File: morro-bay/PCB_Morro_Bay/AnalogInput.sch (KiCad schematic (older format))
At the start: 136 parts, among them SW1 INPUT_RANGE_SEL_1, SW2 INPUT_RANGE_SEL_2, U5 LM2902, U6 LM2902, U7 LM2902, U8 LM2902, U9 LM2902

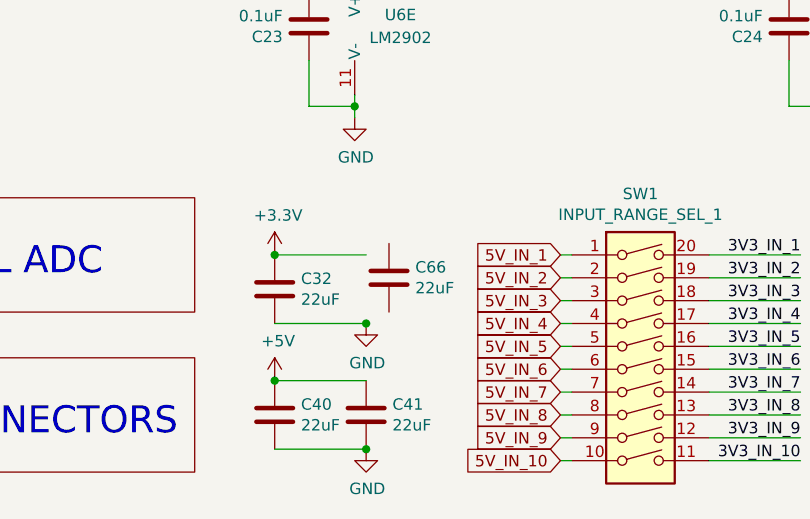
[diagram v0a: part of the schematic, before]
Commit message: Start routing
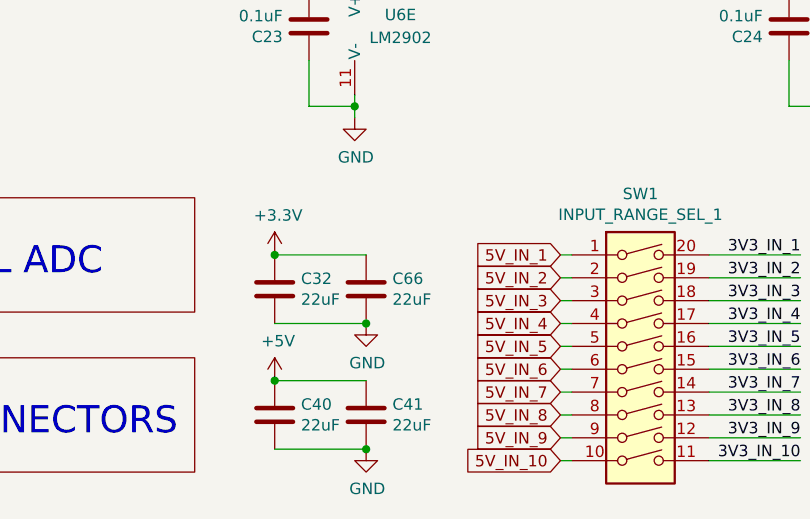
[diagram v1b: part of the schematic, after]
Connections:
- net +3V3: now also C66.1
- net GND: now also C66.2
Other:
- moved on the sheet: C66
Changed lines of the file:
@@
 Wire Wire Line
 	3000 6950 3400 6950
-Connection ~ 3400 6950
 $Comp
 L Device:C C?
@@
 L Device:C C?
 U 1 1 5E88C60F
-P 3500 6750
+P 3400 6800
 AR Path="/5E88C60F" Ref="C?"  Part="1"
 AR Path="/5E59A680/5E88C60F" Ref="C66"  Part="1"
-F 0 "C66" H 3615 6796 50  0000 L CNN
-F 1 "22uF" H 3615 6705 50  0000 L CNN
-F 2 "Capacitor_SMD:C_0805_2012Metric_Pad1.15x1.40mm_HandSolder" H 3538 6600 50  0001 C CNN
-F 3 "~" H 3500 6750 50  0001 C CNN
-F 4 "CL21A226MAQNNNE" H 3500 6750 50  0001 C CNN "Part Number"
-F 5 "https://www.digikey.ca/product-detail/en/samsung-electro-mechanics/CL21A226MAQNNNE/1276-2908-1-ND/3890994" H 3500 6750 50  0001 C CNN "Digikey"
-	1    3500 6750
+F 0 "C66" H 3515 6846 50  0000 L CNN
+F 1 "22uF" H 3515 6755 50  0000 L CNN
+F 2 "Capacitor_SMD:C_0805_2012Metric_Pad1.15x1.40mm_HandSolder" H 3438 6650 50  0001 C CNN
+F 3 "~" H 3400 6800 50  0001 C CNN
+F 4 "CL21A226MAQNNNE" H 3400 6800 50  0001 C CNN "Part Number"
+F 5 "https://www.digikey.ca/product-detail/en/samsung-electro-mechanics/CL21A226MAQNNNE/1276-2908-1-ND/3890994" H 3400 6800 50  0001 C CNN "Digikey"
+	1    3400 6800
 	1    0    0    -1
 $EndComp
@@
 Connection ~ 6950 1800
 Connection ~ 9100 1800
+Connection ~ 3400 6950
 $EndSCHEMATC
